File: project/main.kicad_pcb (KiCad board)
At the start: 6 copper layers, 164 x 254 mm, 191 parts

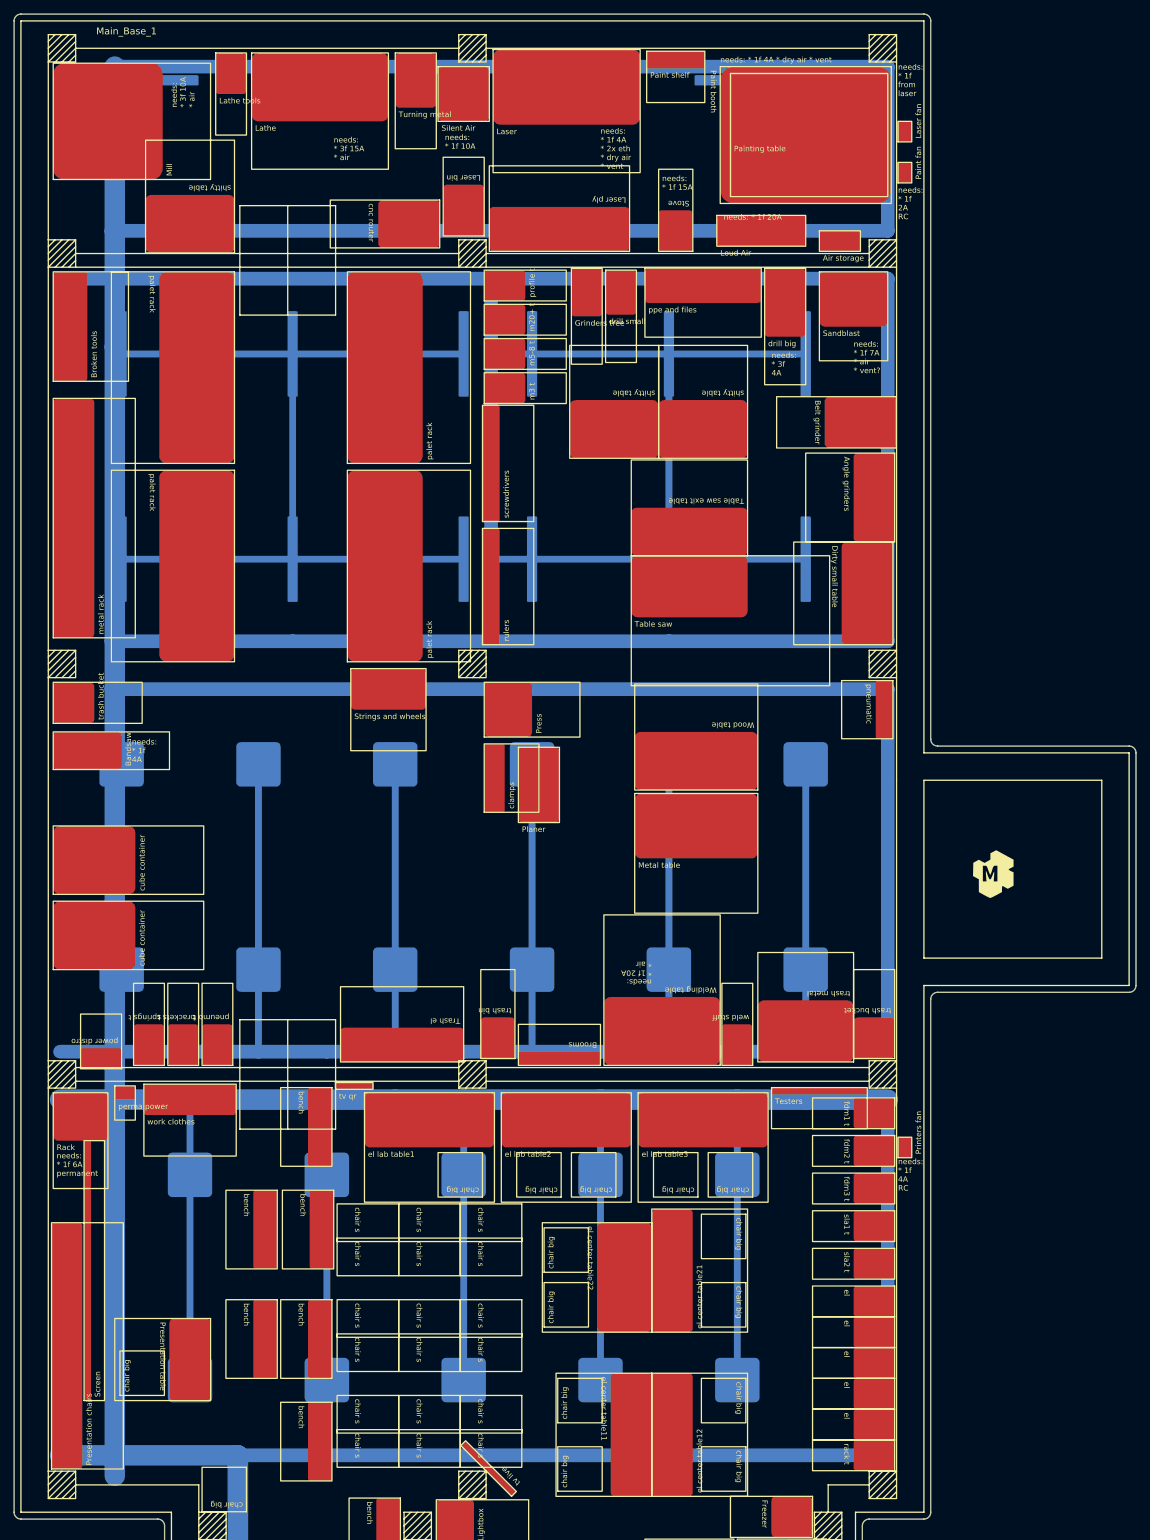
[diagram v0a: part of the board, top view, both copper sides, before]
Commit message: updating main base dimensions
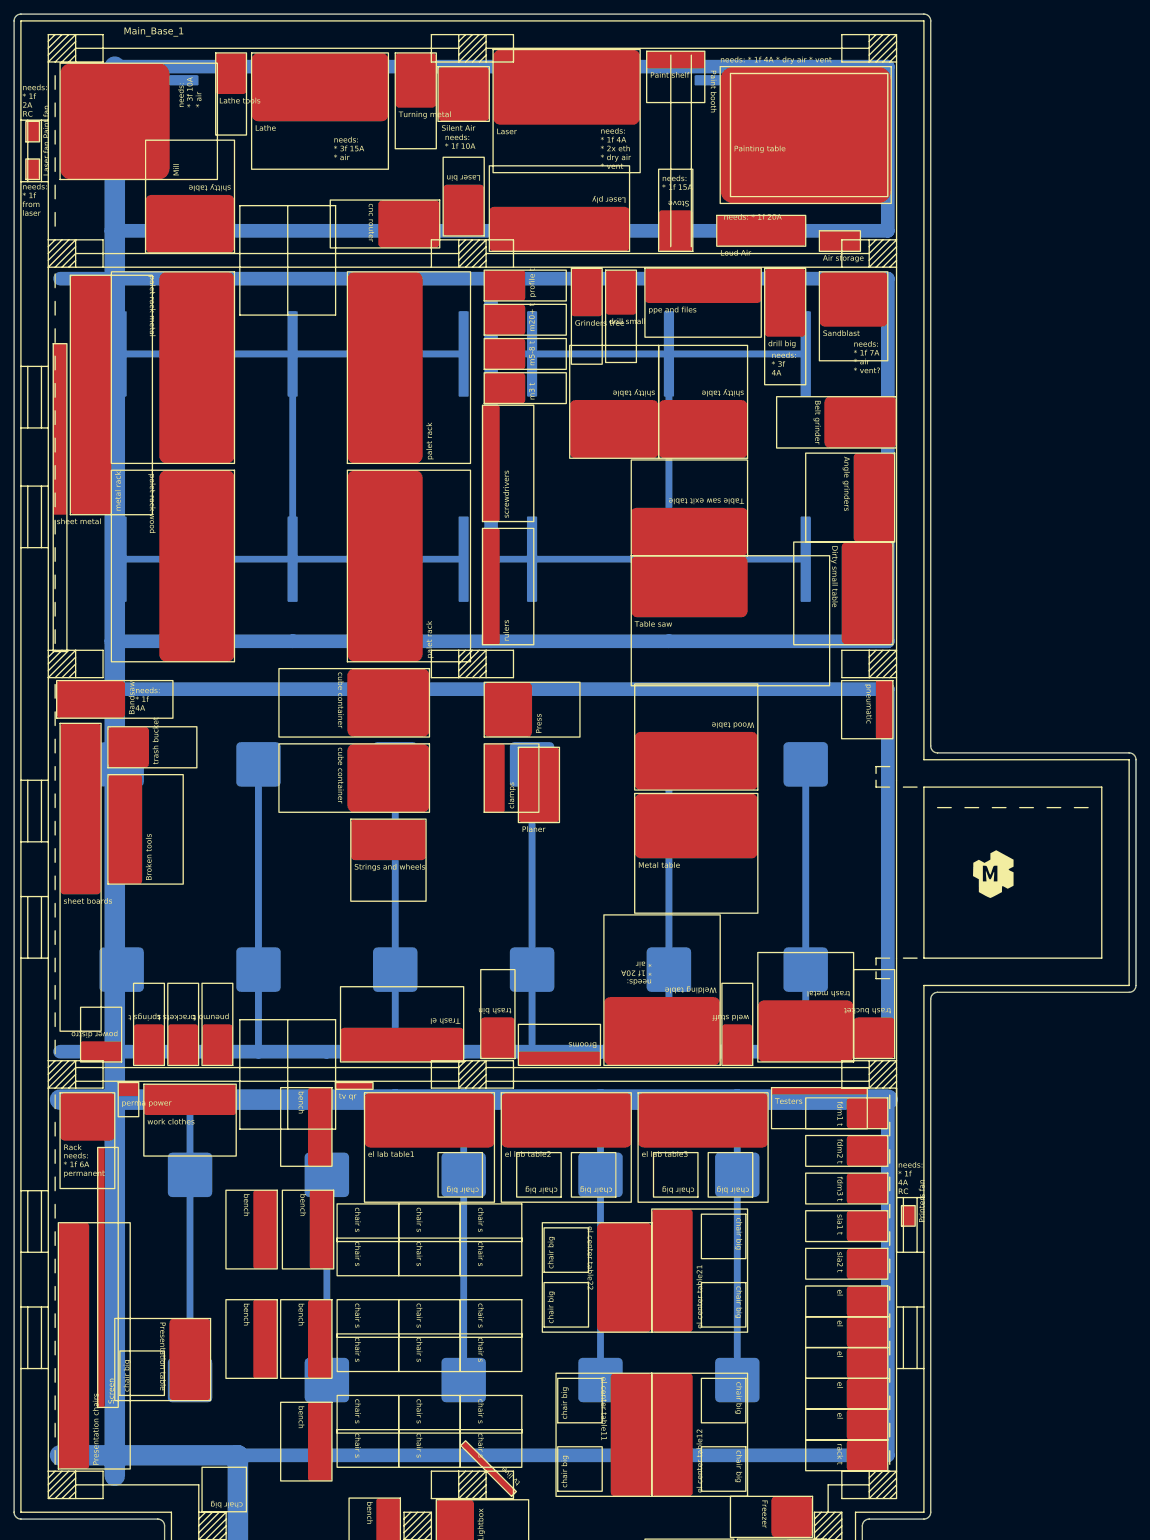
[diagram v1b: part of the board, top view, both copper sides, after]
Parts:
- added R36: sheet boards, -local:_o_sheet_boards__, F.Cu at (81.0, 124.0)
- added R37: sheet metal, -local:_o_sheet_matal__, F.Cu at (80.0, 68.5)
- R41: renamed from R39; value palet rack -> palet rack metal
- R42: renamed from R40; value palet rack -> palet rack wood
- moved R102 127.6 mm to (76.0, 39.0)
- moved R101 127.6 mm to (76.0, 44.5)
- moved R43 73.9 mm to (88.0, 147.5)
- moved R34 64.1 mm to (135.0, 127.0), turned to -90 degrees
- moved R35 64.1 mm to (135.0, 116.0), turned to -90 degrees
- moved R44 22.0 mm to (123.5, 138.0)
- moved R38 18.2 mm to (82.5, 93.5)
- moved R48 10.3 mm to (88.0, 130.5)
- moved R103 10.0 mm to (204.0, 197.5)
- moved R26 7.52 mm to (80.5, 123.2)
- moved R65 2.24 mm to (86.5, 224.0)
- moved R1 1.00 mm to (81.0, 44.5)
- moved R100 1.00 mm to (90.0, 173.5)
- moved R104 1.00 mm to (81.0, 178.0)
- moved R66 1.00 mm to (80.8, 233.0)
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- renumbered R98 to R100, R99 to R101, R100 to R102, R101 to R103, R102 to R104, R36 to R38, R37 to R39, R38 to R40, R41 to R43, R42 to R44, R43 to R45, R44 to R46, R45 to R47, R46 to R48, R47 to R49, R48 to R50, R49 to R51, R50 to R52, R51 to R53, R52 to R54, R53 to R55, R54 to R56, R55 to R57, R56 to R58, R57 to R59, R58 to R60, R59 to R61, R60 to R62, R61 to R63, R62 to R64, R63 to R65, R64 to R66, R65 to R67, R66 to R68, R67 to R69, R68 to R70, R69 to R71, R70 to R72, R71 to R73, R72 to R74, R73 to R75, R74 to R76, R75 to R77, R76 to R78, R77 to R79, R78 to R80, R79 to R81, R80 to R82, R81 to R83, R82 to R84, R83 to R85, R84 to R86, R85 to R87, R86 to R88, R87 to R89, R88 to R90, R89 to R91, R90 to R92, R91 to R93, R92 to R94, R93 to R95, R94 to R96, R95 to R97, R96 to R98, R97 to R99
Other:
- outline, holes or cut-outs redrawn

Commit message: updating main base dimensions and fixing all the things
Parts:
- removed the R99 at (89.5, 176.5)
- added R79: el museum, -local:_e_museum__, F.Cu at (99.3, 254.3)
- added R80: el library, -local:_e_library__, F.Cu at (185.3, 275.3)
- R12: footprint -local:_o_paint_booth__ -> -local:paint_booth
- R14: footprint -local:_o_thin_shelf_single__ -> -local:_o_paint_shelf__
- moved L35 212.4 mm to (148.3, 242.3)
- moved L32 212.4 mm to (116.3, 242.3)
- moved L36 174.4 mm to (148.3, 269.3), turned to 0 degrees
- moved L33 173.6 mm to (178.3, 269.3), turned to 0 degrees
- moved L34 172.7 mm to (178.3, 242.3), turned to 0 degrees
- moved L40 118.9 mm to (94.3, 147.3), turned to 90 degrees
- moved R55 110.9 mm to (99.5, 169.3), turned to 180 degrees
- moved R58 104.6 mm to (104.0, 169.3), turned to 180 degrees
- moved L31 102.8 mm to (191.3, 52.3), turned to 0 degrees
- moved L43 102.5 mm to (164.3, 172.3), turned to 0 degrees
- moved R5 101.6 mm to (143.8, 148.8), turned to 90 degrees
- moved L26 98.7 mm to (96.3, 32.3)
- moved R56 98.3 mm to (108.5, 169.3), turned to 180 degrees
- moved R4 96.4 mm to (102.3, 118.3)
- moved L12 92.8 mm to (111.3, 220.3)
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- renumbered R98 to R100, R100 to R101, R101 to R102, R102 to R103, R103 to R104, R104 to R105, R80 to R81, R81 to R82, R82 to R83, R83 to R84, R84 to R85, R85 to R86, R86 to R87, R79 to R88, R87 to R89, R88 to R90, R89 to R91, R90 to R92, R91 to R93, R92 to R94, R93 to R95, R94 to R96, R95 to R97, R96 to R98, R97 to R99
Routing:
- net Net-(L1-Pad1): track 2248.7 -> 0.00 mm
- net (no net): track 715.6 -> 333.7 mm
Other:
- board size 164 x 254 mm -> 160 x 257 mm

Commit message: fixing electric channel dimensions
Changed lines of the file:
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@@
   (gr_line (start 197.28 178.32) (end 124.28 178.32) (layer "In3.Cu") (width 2))
   (gr_line (start 142.28 118.98) (end 142.28 148.32) (layer "In3.Cu") (width 2))
-  (gr_line (start 82.28 60.32) (end 82.28 114.32) (layer "B.Cu") (width 1.5))
+  (gr_line (start 82.28 60.32) (end 82.28 114.32) (layer "B.Cu") (width 1))
   (gr_line (start 140.28 120.32) (end 140.28 174.32) (layer "B.Cu") (width 0.5))
-  (gr_line (start 82.28 180.32) (end 82.28 234.32) (layer "B.Cu") (width 1.5))
-  (gr_line (start 82.28 174.32) (end 200.28 174.32) (layer "B.Cu") (width 1.5))
-  (gr_line (start 200.28 180.32) (end 200.28 234.32) (layer "B.Cu") (width 1.5))
-  (gr_line (start 200.28 60.32) (end 200.28 114.32) (layer "B.Cu") (width 1.5))
+  (gr_line (start 82.28 180.32) (end 82.28 234.32) (layer "B.Cu") (width 1))
+  (gr_line (start 111.28 174.32) (end 200.28 174.32) (layer "B.Cu") (width 1))
+  (gr_line (start 82.28 174.32) (end 111.28 174.32) (layer "B.Cu") (width 2))
+  (gr_line (start 200.28 180.32) (end 200.28 234.32) (layer "B.Cu") (width 1))
+  (gr_line (start 200.28 60.32) (end 200.28 114.32) (layer "B.Cu") (width 1))
   (gr_line (start 140.28 60.32) (end 140.28 114.32) (layer "B.Cu") (width 0.5))
-  (gr_line (start 82.28 60.32) (end 200.28 60.32) (layer "B.Cu") (width 1.5))
-  (gr_line (start 100.28 247.32) (end 100.28 271.32) (layer "B.Cu") (width 1.5))
-  (gr_line (start 82.28 120.32) (end 200.28 120.32) (layer "B.Cu") (width 1.5))
-  (gr_line (start 82.28 30.32) (end 82.28 54.32) (layer "B.Cu") (width 1.5))
+  (gr_line (start 82.28 60.32) (end 200.28 60.32) (layer "B.Cu") (width 1))
+  (gr_line (start 100.28 247.32) (end 100.28 271.32) (layer "B.Cu") (width 0.5))
+  (gr_line (start 82.28 120.32) (end 200.28 120.32) (layer "B.Cu") (width 1))
+  (gr_line (start 82.28 30.32) (end 82.28 54.32) (layer "B.Cu") (width 1))
   (gr_line (start 167.28 30.32) (end 167.28 54.32) (layer "B.Cu") (width 0.5))
   (gr_line (start 156.28 120.32) (end 156.28 174.32) (layer "B.Cu") (width 0.5))
-  (gr_line (start 200.28 120.32) (end 200.28 174.32) (layer "B.Cu") (width 1.5))
-  (gr_line (start 186.28 271.32) (end 100.28 271.32) (layer "B.Cu") (width 1.5))
-  (gr_line (start 82.28 234.32) (end 200.28 234.32) (layer "B.Cu") (width 1.5))
-  (gr_line (start 82.28 180.32) (end 200.28 180.32) (layer "B.Cu") (width 1.5))
+  (gr_line (start 200.28 120.32) (end 200.28 174.32) (layer "B.Cu") (width 1))
+  (gr_line (start 186.28 271.32) (end 100.28 271.32) (layer "B.Cu") (width 1))
+  (gr_line (start 82.28 234.32) (end 200.28 234.32) (layer "B.Cu") (width 1))
+  (gr_line (start 82.28 180.32) (end 200.28 180.32) (layer "B.Cu") (width 2))
   (gr_line (start 96.28 60.32) (end 96.28 114.32) (layer "B.Cu") (width 0.5))
-  (gr_line (start 186.28 234.32) (end 186.28 274.32) (layer "B.Cu") (width 1.5))
+  (gr_line (start 186.28 234.32) (end 186.28 274.32) (layer "B.Cu") (width 1))
   (gr_line (start 141.28 180.32) (end 141.28 234.32) (layer "B.Cu") (width 0.5))
   (gr_line (start 171.28 60.32) (end 171.28 114.32) (layer "B.Cu") (width 0.5))
@@
   (gr_line (start 186.28 180.32) (end 186.28 234.32) (layer "B.Cu") (width 0.5))
   (gr_line (start 186.28 120.32) (end 186.28 174.32) (layer "B.Cu") (width 0.5))
-  (gr_line (start 111.28 30.32) (end 111.28 276.32) (layer "B.Cu") (width 1.5))
+  (gr_line (start 111.28 30.32) (end 111.28 276.32) (layer "B.Cu") (width 2))
   (gr_line (start 156.28 60.32) (end 156.28 114.32) (layer "B.Cu") (width 0.5))
-  (gr_line (start 82.28 54.32) (end 200.28 54.32) (layer "B.Cu") (width 1.5))
+  (gr_line (start 82.28 54.32) (end 200.28 54.32) (layer "B.Cu") (width 1))
   (gr_line (start 171.28 180.32) (end 171.28 234.32) (layer "B.Cu") (width 0.5))
   (gr_line (start 156.28 180.32) (end 156.28 234.32) (layer "B.Cu") (width 0.5))
   (gr_line (start 186.28 60.32) (end 186.28 114.32) (layer "B.Cu") (width 0.5))
   (gr_line (start 96.28 180.32) (end 96.28 234.32) (layer "B.Cu") (width 0.5))
-  (gr_line (start 200.28 30.32) (end 200.28 54.32) (layer "B.Cu") (width 1.5))
+  (gr_line (start 200.28 30.32) (end 200.28 54.32) (layer "B.Cu") (width 1))
   (gr_line (start 126.28 180.32) (end 126.28 234.32) (layer "B.Cu") (width 0.5))
-  (gr_line (start 82.28 114.32) (end 200.28 114.32) (layer "B.Cu") (width 1.5))
-  (gr_line (start 186.28 240.32) (end 100.28 240.32) (layer "B.Cu") (width 1.5))
-  (gr_line (start 82.28 120.32) (end 82.28 174.32) (layer "B.Cu") (width 1.5))
+  (gr_line (start 82.28 114.32) (end 200.28 114.32) (layer "B.Cu") (width 1))
+  (gr_line (start 186.28 240.32) (end 100.28 240.32) (layer "B.Cu") (width 1))
+  (gr_line (start 82.28 120.32) (end 82.28 174.32) (layer "B.Cu") (width 1))
   (gr_line (start 171.28 120.32) (end 171.28 174.32) (layer "B.Cu") (width 0.5))
-  (gr_line (start 82.28 30.32) (end 200.28 30.32) (layer "B.Cu") (width 1.5))
+  (gr_line (start 82.28 30.32) (end 200.28 30.32) (layer "B.Cu") (width 1))
   (gr_line (start 96.28 120.32) (end 96.28 174.32) (layer "B.Cu") (width 0.5))
   (gr_text "needs:\n* 3f 15A\n* air\n" (at 124.28 40) (layer "F.SilkS")
